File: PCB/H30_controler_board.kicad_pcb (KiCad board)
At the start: 4 copper layers, 80 x 50 mm, 213 parts, among them IC1 MP2338GTL-P, IC2 LTC4359IMS8#PBF, IC3 W25N01GVZEIG, IC4 ADS1115IDGSR, IC5 ADS1115IDGSR, IC6 DRV8833CPWPR, J1 662102145021, J10 653004114822, J11 653006114822, J12 653002114822, J14 653006114822, J15 XT60_YELLOW, J16 653002114822, J18 653102131822, J19 653102131822, J2 USB_C_Receptacle_USB2.0_14P, J20 653003114822, J21 653003114822, J22 653003114822, J23 653003114822, J24 653003114822, J25 653003114822, J26 653003114822, J27 653003114822, J28 653006114822, J29 Conn_02x07_Odd_Even, J3 SWD, J30 Conn_01x14_Socket, J4 653004114822, J5 653004114822, J6 653004114822, J7 653002114822, J8 TC2030, J9 653004114822, Q1 AO3401A, Q10 PSMNR56-25YLEX, Q11 2N7002, Q12 PSMNR56-25YLEX, Q13 SI2301-TP, Q2 SI2301-TP, Q3 2N7002, Q4 PSMNR56-25YLEX, Q5 PSMNR56-25YLEX, Q6 SI2301-TP, Q7 PSMNR56-25YLEX, Q8 2N7002, Q9 SI2301-TP, SW1 SW_Nidec_CAS-120A1, SW3 SW_Nidec_CAS-120A1, U1 STM32L476RCTx, U2 USBLC6-2SC6, Y1 16MHz

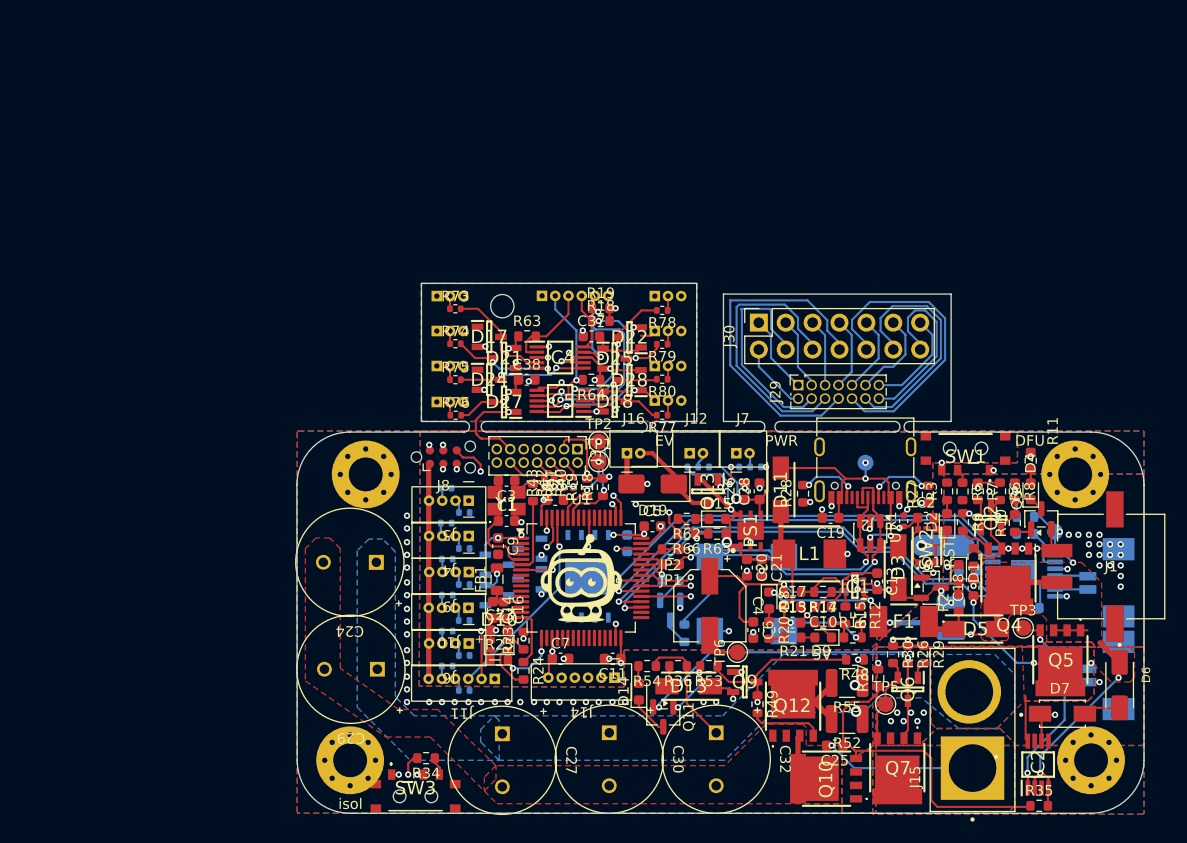
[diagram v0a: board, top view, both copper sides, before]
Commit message: PCB V1.1
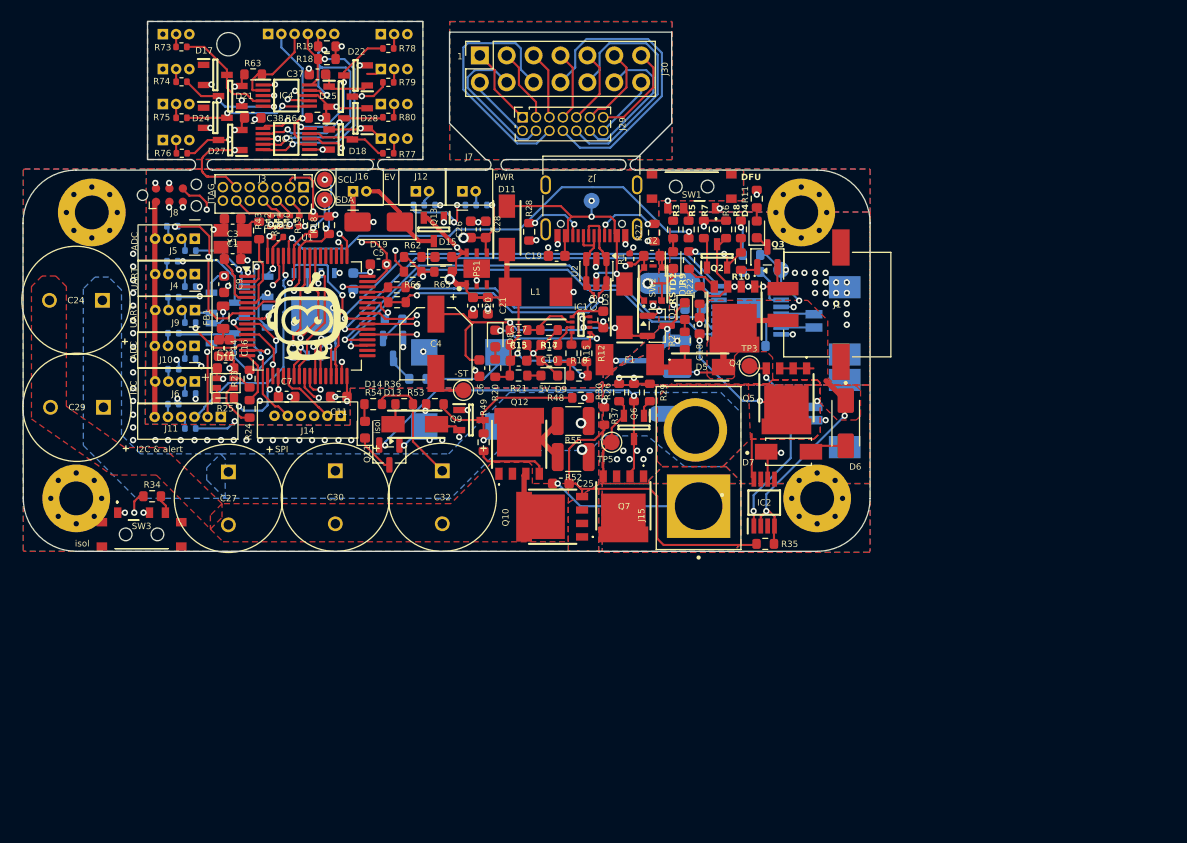
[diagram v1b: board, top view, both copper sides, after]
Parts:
- C8: footprint Capacitor_SMD:C_0603_1608Metric -> Capacitor_SMD:C_0402_1005Metric
- moved J30 36.5 mm to (108.2, 38.5)
- moved J29 36.3 mm to (112.2, 44.4)
- moved C8 36.1 mm to (89.2, 55.7)
- moved Q8 36.0 mm to (100.0, 66.2)
- moved R32 36.0 mm to (100.1, 63.5)
- moved H1 35.8 mm to (138.6, 53.4)
- moved H2 35.8 mm to (140.1, 80.3)
- moved IC6 35.8 mm to (133.7, 62.6)
- moved J15 35.8 mm to (128.9, 77.5)
- moved J19 35.8 mm to (142.6, 63.6)
- moved R22 35.8 mm to (129.0, 61.1)
- moved SW1 35.8 mm to (128.2, 50.9)
- moved C18 35.8 mm to (129.0, 64.0)
- moved IC2 35.8 mm to (135.1, 80.8)
- moved J1 35.8 mm to (142.0, 62.0)
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- renumbered TP6 to -ST, TP2 to SCL, TP1 to SDA
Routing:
- net /BOOT0: track 0.00 -> 44.5 mm, vias 0 -> 2
- net /I2C1_SCL: track 33.5 -> 63.3 mm, vias 4 -> 8
- net /I2C1_SDA: track 32.6 -> 60.7 mm, vias 5 -> 8
- net -ST: track 69.1 -> 94.8 mm, vias 34 -> 43
- net /USART3_RX: track 0.00 -> 23.1 mm, vias 0 -> 2
- net /ADC1_IN1+: track 0.00 -> 20.7 mm, vias 0 -> 2
- net /USART3_TX: track 0.00 -> 20.6 mm, vias 0 -> 2
- net /SPI1_CS: track 0.00 -> 18.1 mm, vias 0 -> 2
- net /ADC3_IN3+: track 0.00 -> 17.2 mm, vias 0 -> 1
- net /SPI1_MISO: track 0.00 -> 16.7 mm, vias 0 -> 1
- net /SPI1_MOSI: track 0.00 -> 15.8 mm, vias 0 -> 1
- net /QUADSPI_NCS: track 0.00 -> 15.3 mm, vias 0 -> 1
- net /ADC1_IN2-: track 0.00 -> 14.5 mm, vias 0 -> 2
- net /UART4_RX: track 0.00 -> 13.0 mm, vias 0 -> 2
- net /14: track 17.3 -> 6.06 mm
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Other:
- outline, holes or cut-outs redrawn
- board text added: "1"
- board text added: "ADC"
- board text added: "Adapatateur 1mm 2.56mm"
- board text added: "I2C"
- board text added: "I2C & alert"
- board text added: "JTAG"
- board text added: "SPI"
- board text added: "UART"
